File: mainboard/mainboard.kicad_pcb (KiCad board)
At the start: 2 copper layers, 53 x 53 mm, 95 parts, among them J1 USB_B_Micro, J2 Conn_01x19_MountingPin, J3 Conn_01x19_MountingPin, J4 Conn_01x02_Male, Q1 DMG2301L, Q2 MMBT3904, Q3 MMBT3904, SW1 SW_Push, SW2 SW_Push, U1 ESP32-WROOM-32, U2 tps63070, U3 tps63070, U4 tps63070, U5 CP2102N-A01-GQFN24, U6 BME680, U7 BH1750FVI, U8 LIS3MDL, U9 ADXL343

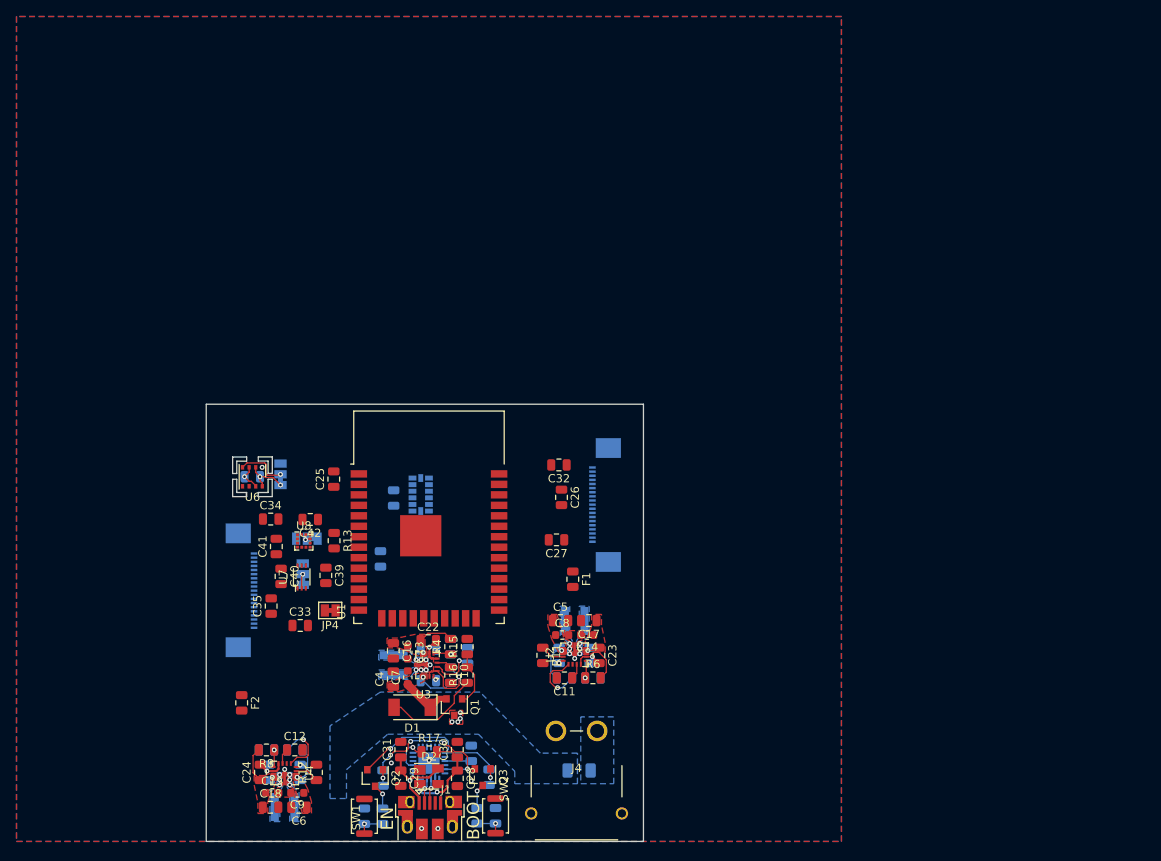
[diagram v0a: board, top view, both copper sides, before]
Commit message: More WIP
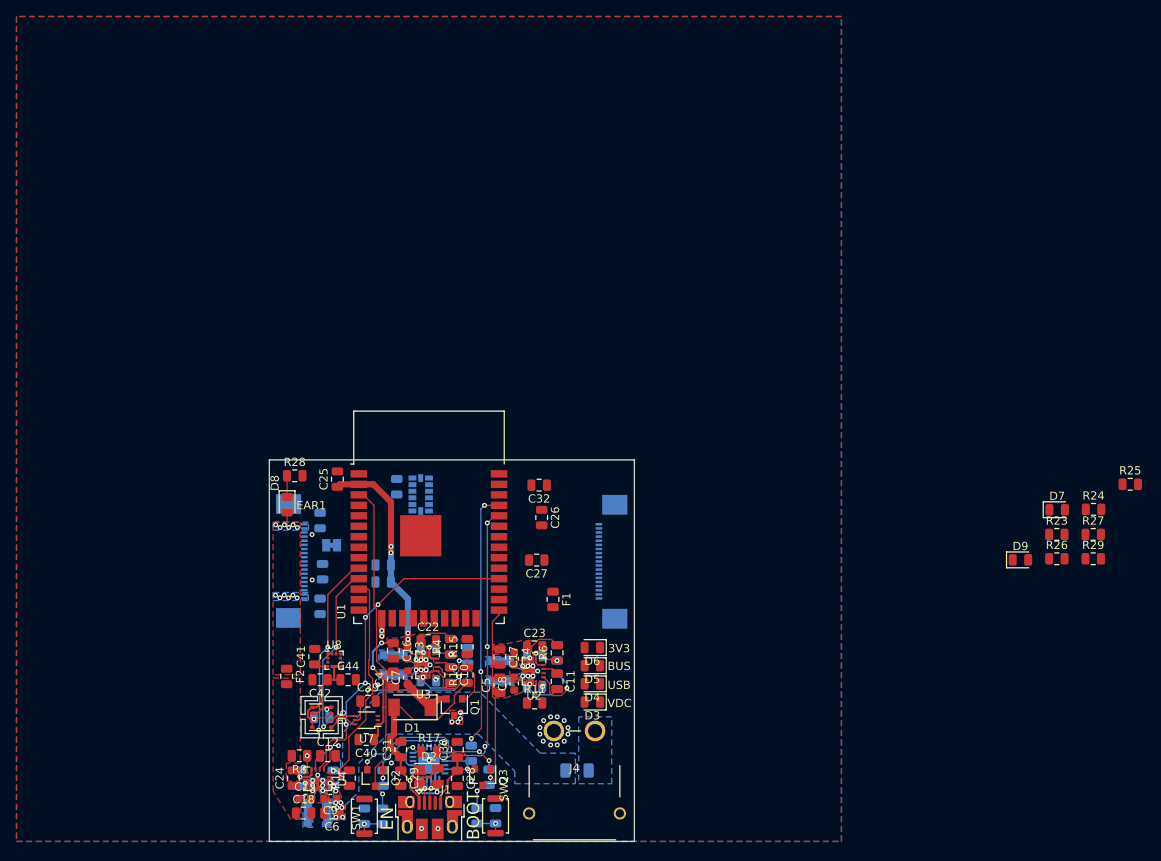
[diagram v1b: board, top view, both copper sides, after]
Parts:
- removed JP1, JP2, JP3: Jumper_3_Bridged12, Jumper:SolderJumper-3_P1.3mm_Bridged12_Pad1.0x1.5mm
- added C44: 1 uC, Capacitor_SMD:C_0805_2012Metric, F.Cu at (70.2, 110.4)
- added D3: LED, LED_SMD:LED_0805_2012Metric, F.Cu at (99.8, 113.1)
- added D4: LED, LED_SMD:LED_0805_2012Metric, F.Cu at (99.8, 110.9)
- added D5: LED, LED_SMD:LED_0805_2012Metric, F.Cu at (99.8, 108.7)
- added D6: LED, LED_SMD:LED_0805_2012Metric, F.Cu at (99.8, 106.5)
- added D7: LED, LED_SMD:LED_0805_2012Metric, F.Cu at (156.2, 89.8)
- added D8: LED, LED_SMD:LED_0805_2012Metric, F.Cu at (62.8, 89.2)
- added D9: LED, LED_SMD:LED_0805_2012Metric, F.Cu at (151.7, 95.9)
- added R23: 1 kR, Resistor_SMD:R_0805_2012Metric, F.Cu at (156.1, 92.8)
- added R24: 330 R, Resistor_SMD:R_0805_2012Metric, F.Cu at (160.6, 89.7)
- added R25: 1 kR, Resistor_SMD:R_0805_2012Metric, F.Cu at (165.0, 86.7)
- added R26: 220 R, Resistor_SMD:R_0805_2012Metric, F.Cu at (156.1, 95.7)
- added R27: 470 R, Resistor_SMD:R_0805_2012Metric, F.Cu at (160.5, 92.8)
- added R28: 470 R, Resistor_SMD:R_0805_2012Metric, F.Cu at (63.7, 85.7)
- added R29: 220 R, Resistor_SMD:R_0805_2012Metric, F.Cu at (160.5, 95.7)
- C33, C34, C35, JP4, R13: moved to B.Cu
- moved C38 30.4 mm to (67.0, 115.0)
- moved U6 30.3 mm to (67.0, 114.9), turned to 270 degrees
- moved C40 22.3 mm to (72.4, 117.7), turned to 180 degrees
- moved C42 19.5 mm to (66.8, 110.4)
- moved U7 19.1 mm to (72.4, 115.3), turned to 180 degrees
- moved C39 16.1 mm to (72.6, 113.0), turned to 0 degrees
- moved U8 14.9 mm to (68.5, 108.0)
- moved C41 14.1 mm to (66.2, 107.6)
- moved C17 11.7 mm to (88.6, 107.6), turned to 270 degrees
- moved L2 10.9 mm to (88.6, 109.3), turned to 90 degrees
- moved C5 10.7 mm to (88.6, 111.1), turned to 90 degrees
- moved C14 9.29 mm to (90.3, 107.8), turned to 270 degrees
- moved C8 8.27 mm to (90.3, 110.9), turned to 90 degrees
- moved JP4 7.90 mm to (68.2, 94.1)
- moved C23 7.87 mm to (92.8, 106.4), turned to 0 degrees
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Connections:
- U1 pad 26: Net-(U1-Pad26) -> /IO4
- U6 pad 5: Net-(JP2-Pad2) -> +3V3
- U7 pad 2: Net-(JP1-Pad2) -> GND
- U8 pad 9: Net-(JP3-Pad2) -> GND
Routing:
- net +3V3: track 7.58 -> 60.3 mm, vias 3 -> 8
- net /PG_VCC1: track 0.00 -> 39.7 mm, vias 0 -> 4
- net /EN: track 3.07 -> 40.6 mm
- net /RXD: track 0.00 -> 34.8 mm, vias 0 -> 3
- net /TXD: track 0.00 -> 32.2 mm, vias 0 -> 3
- net /SCL: track 0.00 -> 28.6 mm, vias 0 -> 2
- net /VCC1_EN: track 2.90 -> 28.7 mm
- net /SDA: track 0.00 -> 25.3 mm, vias 0 -> 2
- net /IO0: track 3.02 -> 25.8 mm
- net /PG_3V3: track 5.72 -> 24.6 mm, vias 1 -> 2
- net VUSB: track 24.0 -> 30.8 mm
- net Net-(JP2-Pad2): track 6.41 -> 0.00 mm, vias 1 -> 0
- net Net-(C15-Pad1): track 4.31 -> 0.00 mm
- net Net-(D8-Pad1): track 0.00 -> 2.57 mm
- net Net-(R3-Pad1): track 7.14 -> 4.64 mm
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- added copper zone on B.Cu, net VCC_EAR1
- added copper zone on F.Cu, net VCC_EAR1
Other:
- board size 53 x 53 mm -> 44.3 x 46.2 mm
- board text added: "3V3"
- board text added: "BUS"
- board text added: "EAR1"
- board text added: "USB"
- board text added: "VDC"
